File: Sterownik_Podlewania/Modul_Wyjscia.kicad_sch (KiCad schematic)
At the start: 7 parts, among them J2 Screw_Terminal_01x02, K2 SANYOU_SRD_Form_C, Q2 BC547

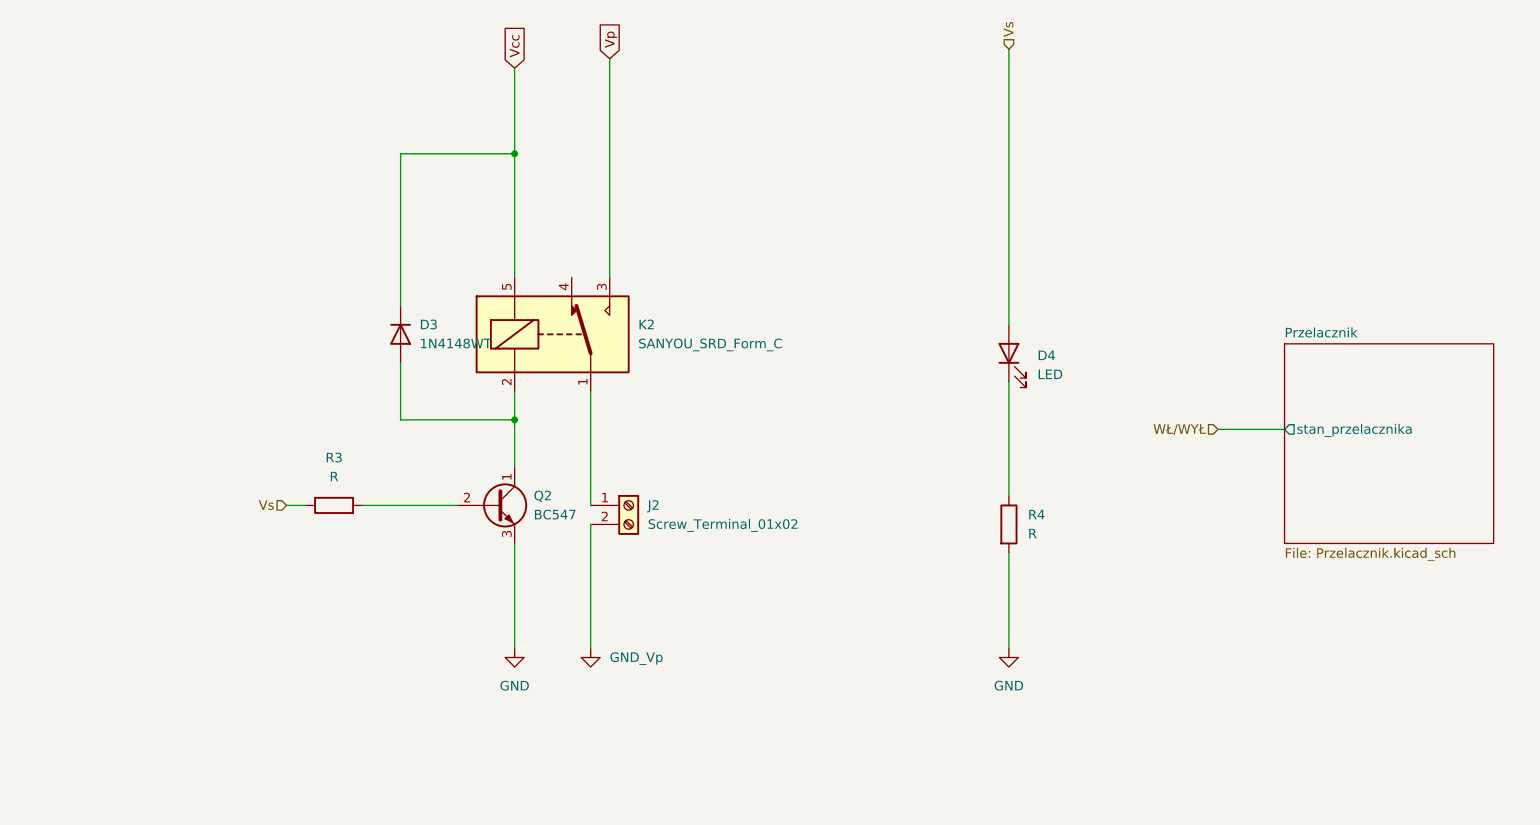
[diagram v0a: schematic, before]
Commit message: Poprawki estetyczne schematu
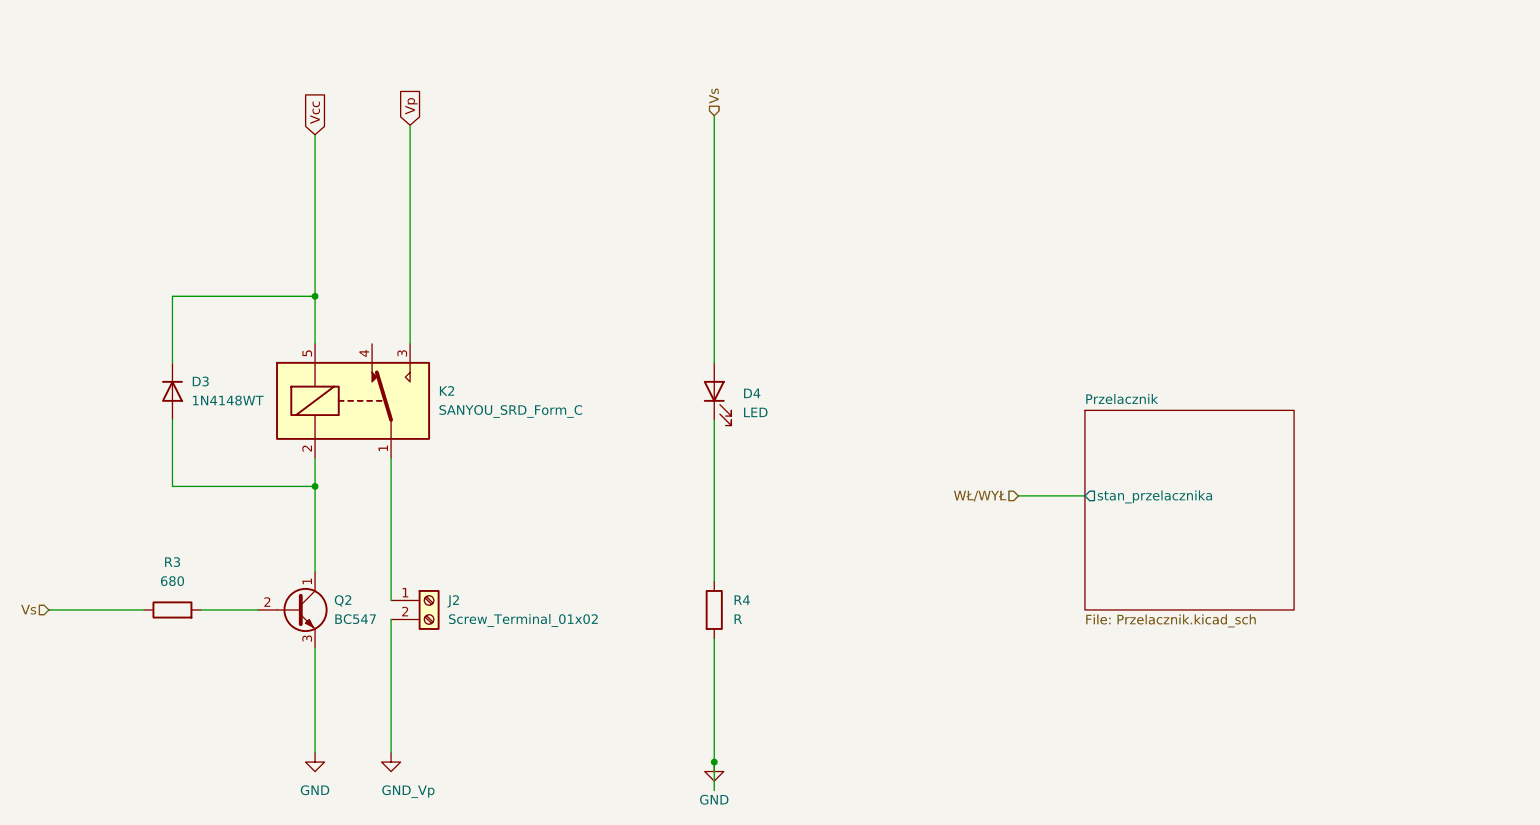
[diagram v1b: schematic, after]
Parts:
- R3: value R -> 680
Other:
- moved on the sheet: D3, D4, J2, K2, Q2, R3, R4
